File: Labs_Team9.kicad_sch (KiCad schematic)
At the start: 51 parts, among them J1 Conn_02x04_Counter_Clockwise, J2 Conn_01x03_Pin, J3 Conn_01x04_Pin, J4 Conn_01x04_Pin, J5 USB_C_Receptacle_PowerOnly_6P, SW1 SW_Push, SW2 SW_Push, SW3 SW_Push, SW4 SW_Push, SW5 SW_Push, SW6 SW_Push, U1 STM32F411RETx, U2 TLV62569DBV, Y1 Crystal_GND24

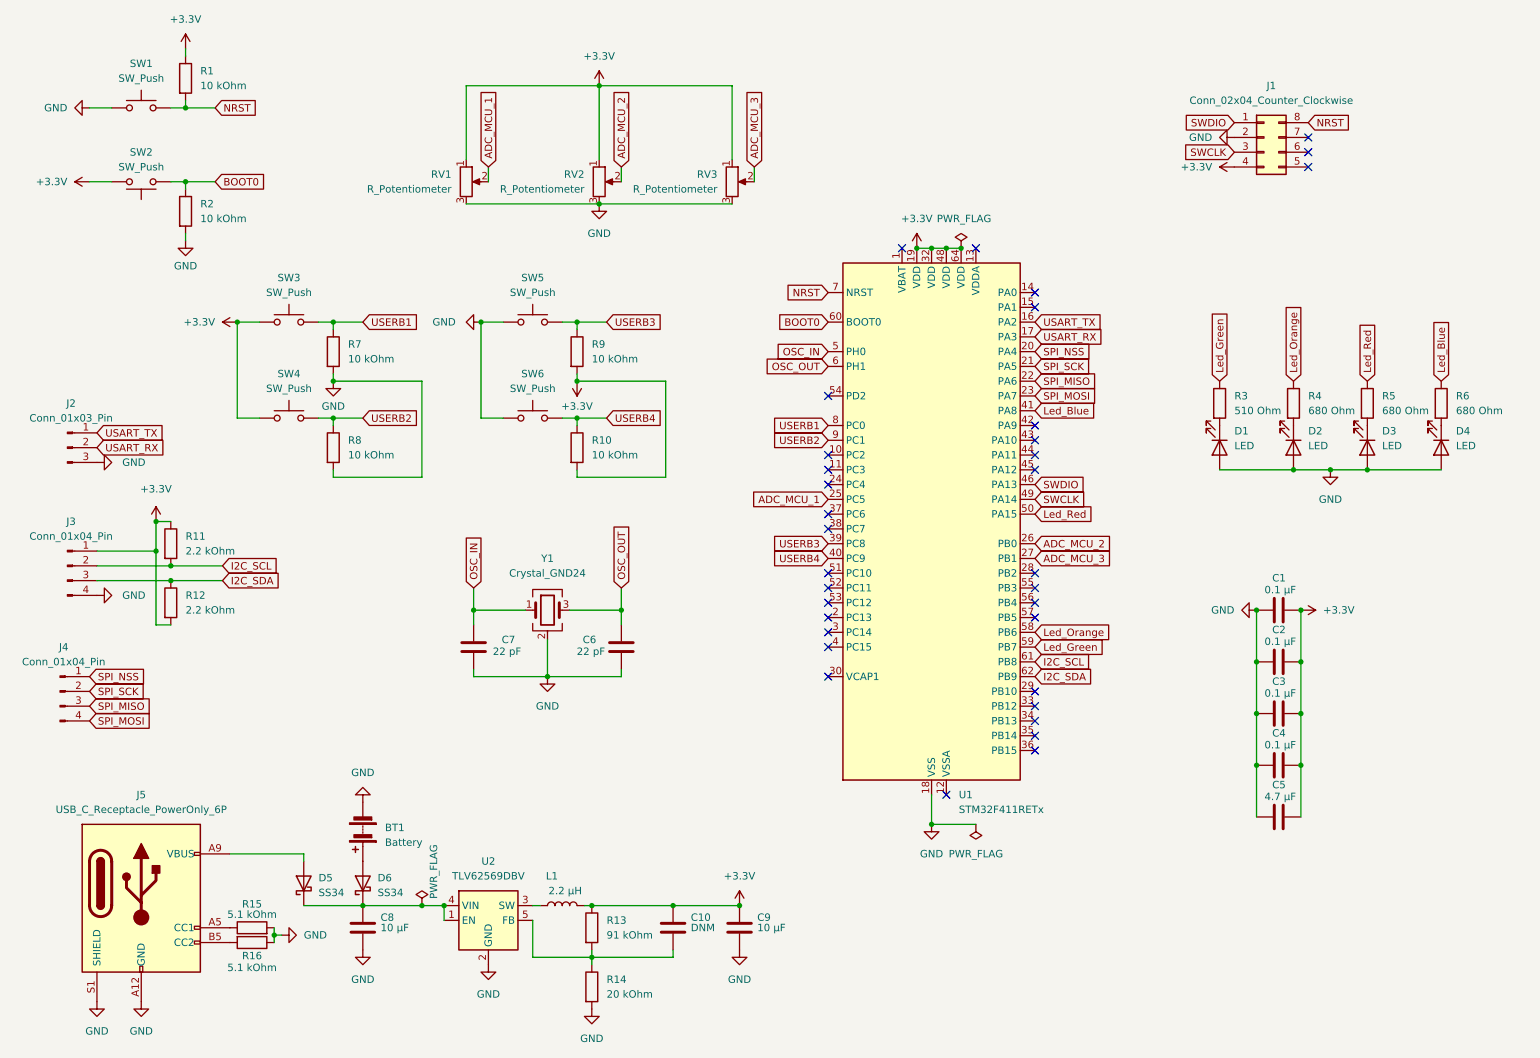
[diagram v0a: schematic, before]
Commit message: lab5: add part of the schematic
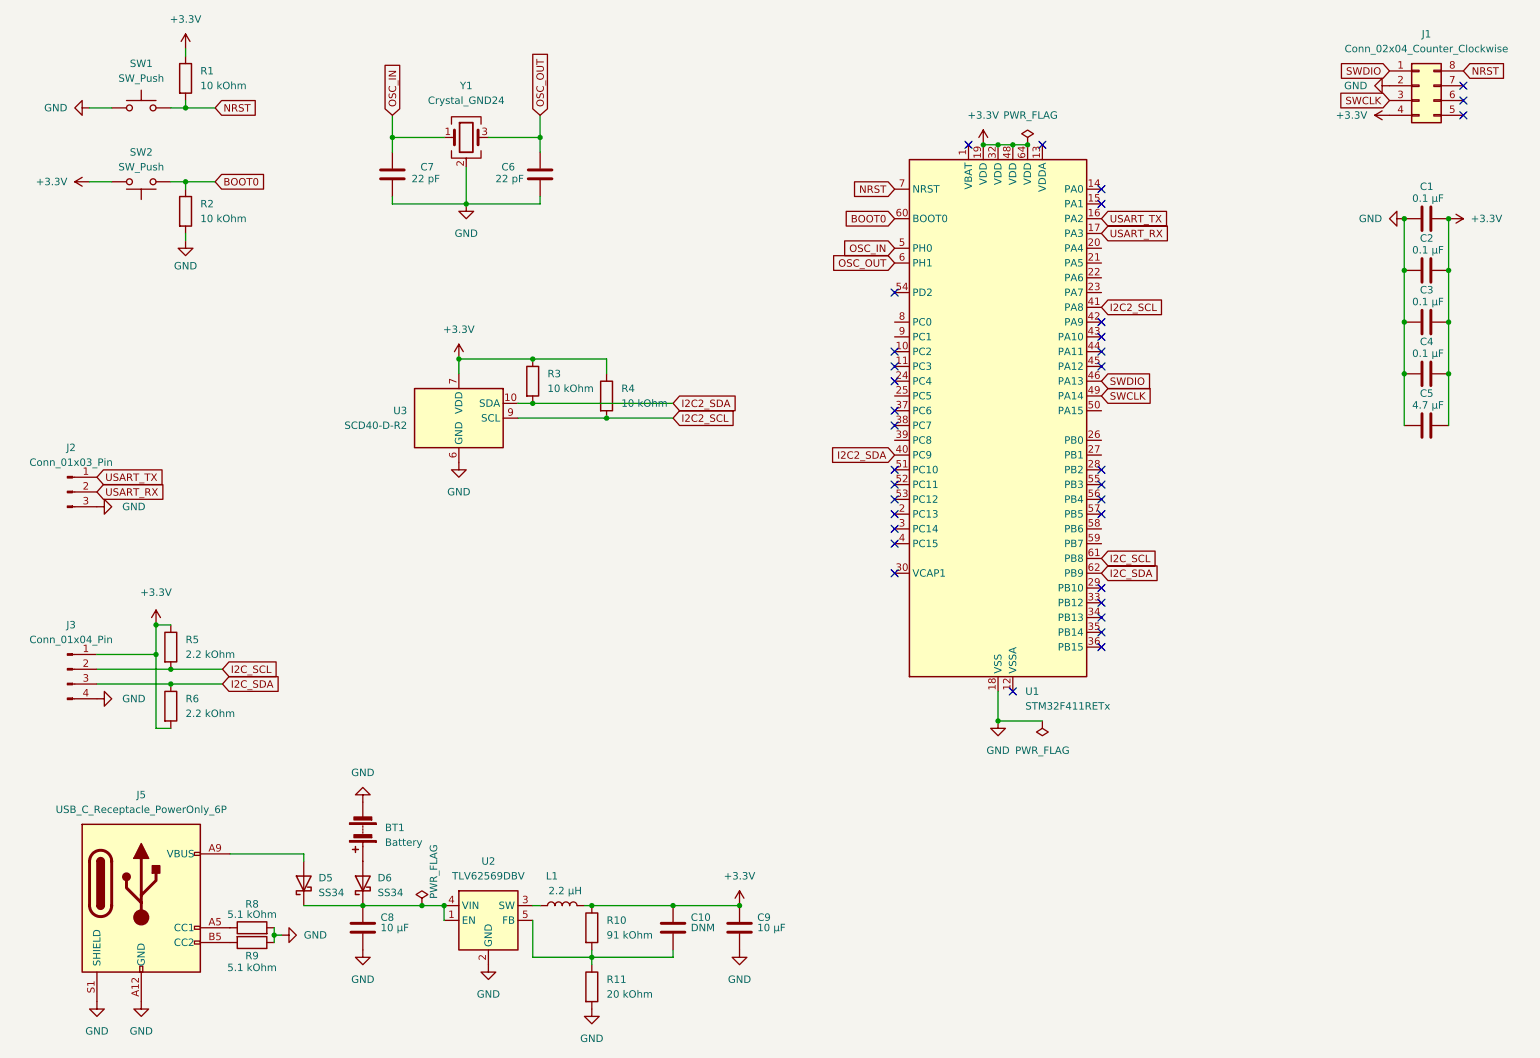
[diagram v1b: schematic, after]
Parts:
- removed D1, D2, D3, D4: LED, LED_SMD:LED_1206_3216Metric_Pad1.42x1.75mm_HandSolder, symbol Device:LED
- removed J4: Conn_01x04_Pin, Connector_PinHeader_2.54mm:PinHeader_1x04_P2.54mm_Vertical, symbol Connector:Conn_01x04_Pin
- removed R10, R7, R8, R9: 10 kOhm, Resistor_SMD:R_1206_3216Metric_Pad1.30x1.75mm_HandSolder, symbol Device:R
- removed R5, R6: 680 Ohm, Resistor_SMD:R_1206_3216Metric_Pad1.30x1.75mm_HandSolder, symbol Device:R
- removed RV1, RV2, RV3: R_Potentiometer, Potentiometer_THT:Potentiometer_Bourns_3339P_Vertical_HandSoldering, symbol Device:R_Potentiometer
- removed SW3, SW4, SW5, SW6: SW_Push, Buttons_Switches_THT:SW_PUSH_6mm, symbol Switch:SW_Push
- added U3: SCD40-D-R2, Sensor:Sensirion_SCD4x-1EP_10.1x10.1mm_P1.25mm_EP4.8x4.8mm, symbol Sensor_Gas:SCD40-D-R2
- R3: value 510 Ohm -> 10 kOhm
- R4: value 680 Ohm -> 10 kOhm
- renumbered R13 to R10, R14 to R11, R11 to R5, R12 to R6, R15 to R8, R16 to R9
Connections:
- net Led_Blue is gone; now on net I2C2_SCL: U1.41 (PA8)
- net USERB4 is gone; now on net I2C2_SDA: U1.40 (PC9)
- net +3.3V: now also R3.1, R4.1, U3.19 (VDD), U3.7 (VDD)
- net GND: now also U3.20 (GND), U3.21 (GND), U3.6 (GND)
- net I2C2_SDA: now reaches R3.2
- net I2C2_SDA: now also U3.10 (SDA)
- net I2C2_SCL: now reaches R4.2
- net I2C2_SCL: now also U3.9 (SCL)
- net ADC_MCU_1: no longer names the net of U1.25 (PC5)
- net ADC_MCU_2: no longer names the net of U1.26 (PB0)
- net ADC_MCU_3: no longer names the net of U1.27 (PB1)
- net Led_Green: no longer names the net of U1.59 (PB7)
- net Led_Green: no longer R3.1
- net Led_Orange: no longer names the net of U1.58 (PB6)
- net Led_Orange: no longer R4.1
- net Led_Red: no longer names the net of U1.50 (PA15)
- net SPI_MISO: no longer names the net of U1.22 (PA6)
- net SPI_MOSI: no longer names the net of U1.23 (PA7)
- net SPI_NSS: no longer names the net of U1.20 (PA4)
- net SPI_SCK: no longer names the net of U1.21 (PA5)
- net USERB1: no longer names the net of U1.8 (PC0)
- net USERB2: no longer names the net of U1.9 (PC1)
- net USERB3: no longer names the net of U1.39 (PC8)
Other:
- moved on the sheet: C1, C2, C3, C4, C5, C6, C7, J1, J2, J3, R5, R6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
